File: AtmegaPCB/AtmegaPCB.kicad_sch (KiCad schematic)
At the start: 19 parts

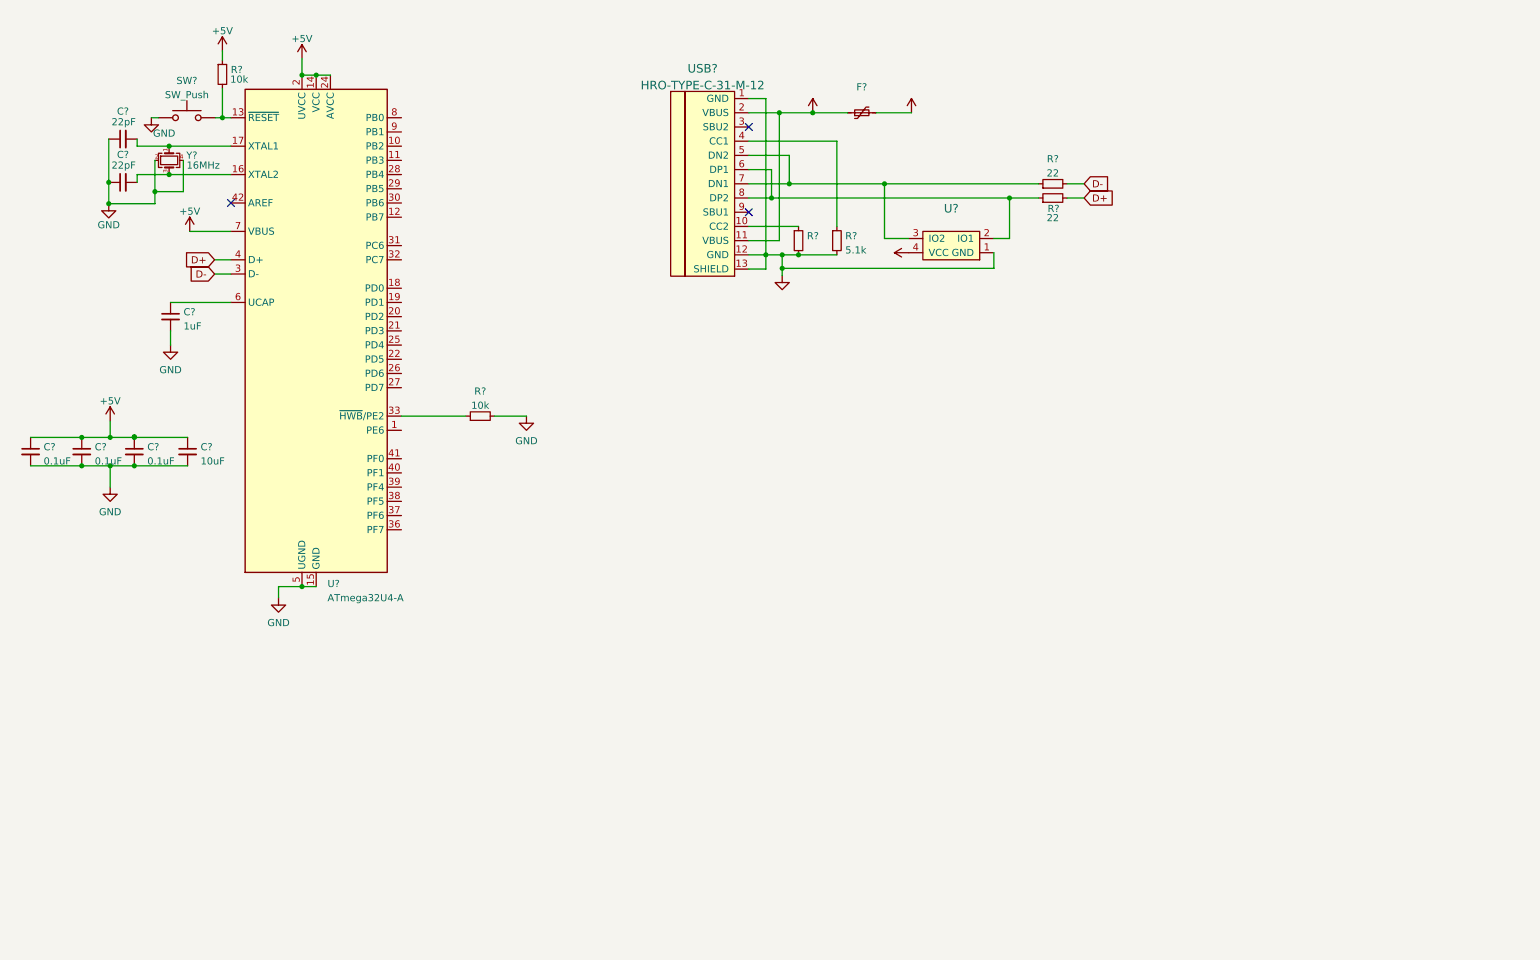
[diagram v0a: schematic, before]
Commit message: Matrix done!
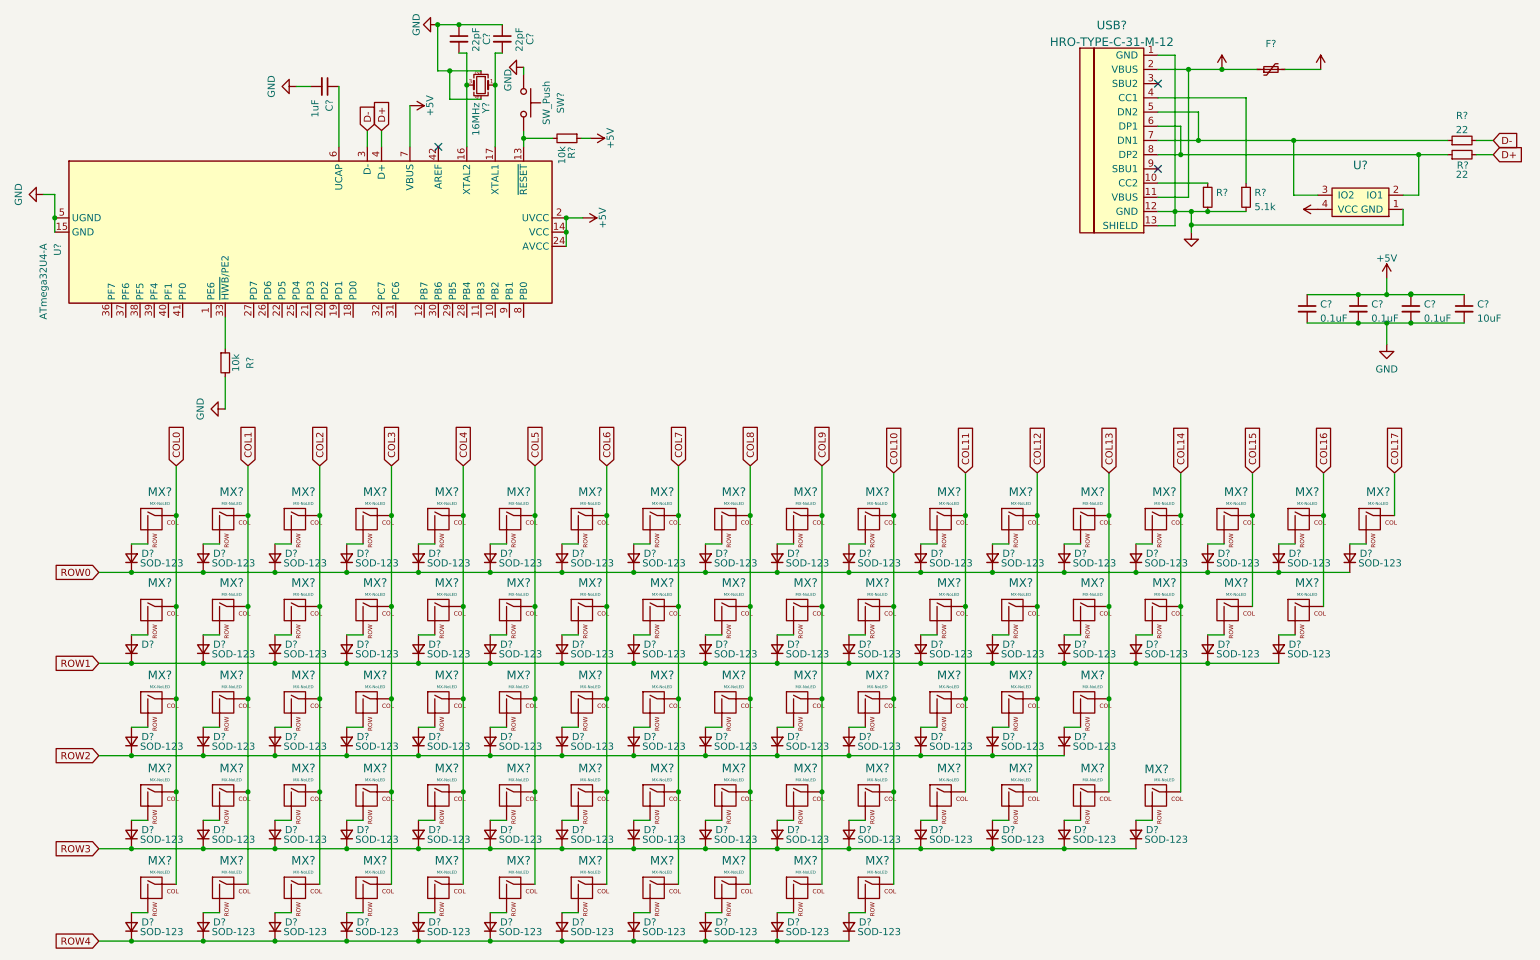
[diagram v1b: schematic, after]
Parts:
- added D? (x74): SOD-123, symbol Device:D_Small
- added D?: (no value), symbol Device:D_Small
- added MX? (x74): MX-NoLED, symbol MX_Alps_Hybrid:MX-NoLED
- added MX?: (no value), symbol MX_Alps_Hybrid:MX-NoLED
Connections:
- new net: D?.2 (A), MX?.2 (ROW) (x75)
- new net COL0: MX?.1 (COL), MX?.1 (COL), MX?.1 (COL), MX?.1 (COL), MX?.1 (COL)
- new net COL1: MX?.1 (COL), MX?.1 (COL), MX?.1 (COL), MX?.1 (COL), MX?.1 (COL)
- new net COL10: MX?.1 (COL), MX?.1 (COL), MX?.1 (COL), MX?.1 (COL), MX?.1 (COL)
- new net COL11: MX?.1 (COL), MX?.1 (COL), MX?.1 (COL), MX?.1 (COL)
- new net COL12: MX?.1 (COL), MX?.1 (COL), MX?.1 (COL), MX?.1 (COL)
- new net COL13: MX?.1 (COL), MX?.1 (COL), MX?.1 (COL), MX?.1 (COL)
- new net COL14: MX?.1 (COL), MX?.1 (COL), MX?.1 (COL)
- new net COL15: MX?.1 (COL), MX?.1 (COL)
- new net COL16: MX?.1 (COL), MX?.1 (COL)
- new net COL17: MX?.1 (COL)
- new net COL2: MX?.1 (COL), MX?.1 (COL), MX?.1 (COL), MX?.1 (COL), MX?.1 (COL)
- new net COL3: MX?.1 (COL), MX?.1 (COL), MX?.1 (COL), MX?.1 (COL), MX?.1 (COL)
- new net COL4: MX?.1 (COL), MX?.1 (COL), MX?.1 (COL), MX?.1 (COL), MX?.1 (COL)
- new net COL5: MX?.1 (COL), MX?.1 (COL), MX?.1 (COL), MX?.1 (COL), MX?.1 (COL)
- new net COL6: MX?.1 (COL), MX?.1 (COL), MX?.1 (COL), MX?.1 (COL), MX?.1 (COL)
- new net COL7: MX?.1 (COL), MX?.1 (COL), MX?.1 (COL), MX?.1 (COL), MX?.1 (COL)
- new net COL8: MX?.1 (COL), MX?.1 (COL), MX?.1 (COL), MX?.1 (COL), MX?.1 (COL)
- new net COL9: MX?.1 (COL), MX?.1 (COL), MX?.1 (COL), MX?.1 (COL), MX?.1 (COL)
- new net ROW0: D?.1 (K), D?.1 (K), D?.1 (K), D?.1 (K), D?.1 (K), D?.1 (K), D?.1 (K), D?.1 (K), D?.1 (K), D?.1 (K), D?.1 (K), D?.1 (K), D?.1 (K), D?.1 (K), D?.1 (K), D?.1 (K), D?.1 (K), D?.1 (K)
- new net ROW1: D?.1 (K), D?.1 (K), D?.1 (K), D?.1 (K), D?.1 (K), D?.1 (K), D?.1 (K), D?.1 (K), D?.1 (K), D?.1 (K), D?.1 (K), D?.1 (K), D?.1 (K), D?.1 (K), D?.1 (K), D?.1 (K), D?.1 (K)
- new net ROW2: D?.1 (K), D?.1 (K), D?.1 (K), D?.1 (K), D?.1 (K), D?.1 (K), D?.1 (K), D?.1 (K), D?.1 (K), D?.1 (K), D?.1 (K), D?.1 (K), D?.1 (K), D?.1 (K)
- new net ROW3: D?.1 (K), D?.1 (K), D?.1 (K), D?.1 (K), D?.1 (K), D?.1 (K), D?.1 (K), D?.1 (K), D?.1 (K), D?.1 (K), D?.1 (K), D?.1 (K), D?.1 (K), D?.1 (K), D?.1 (K)
- new net ROW4: D?.1 (K), D?.1 (K), D?.1 (K), D?.1 (K), D?.1 (K), D?.1 (K), D?.1 (K), D?.1 (K), D?.1 (K), D?.1 (K), D?.1 (K)
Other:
- moved on the sheet: C?, F?, R?, SW?, U?, USB?, Y?
